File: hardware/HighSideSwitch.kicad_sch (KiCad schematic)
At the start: 5 parts, among them Q901 MMBTA42

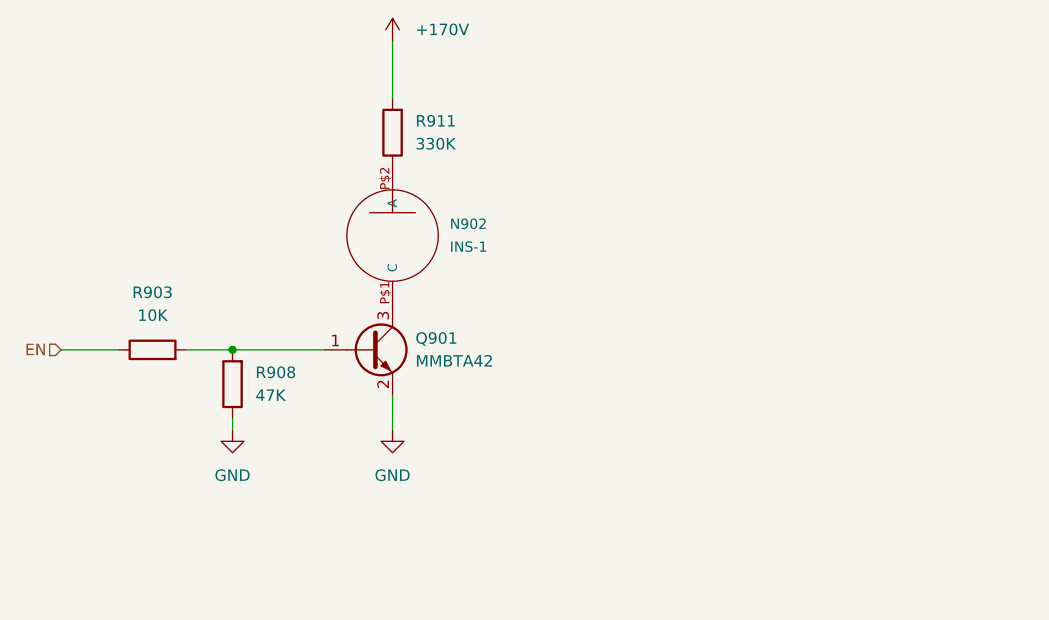
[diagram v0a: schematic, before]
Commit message: 2/static version
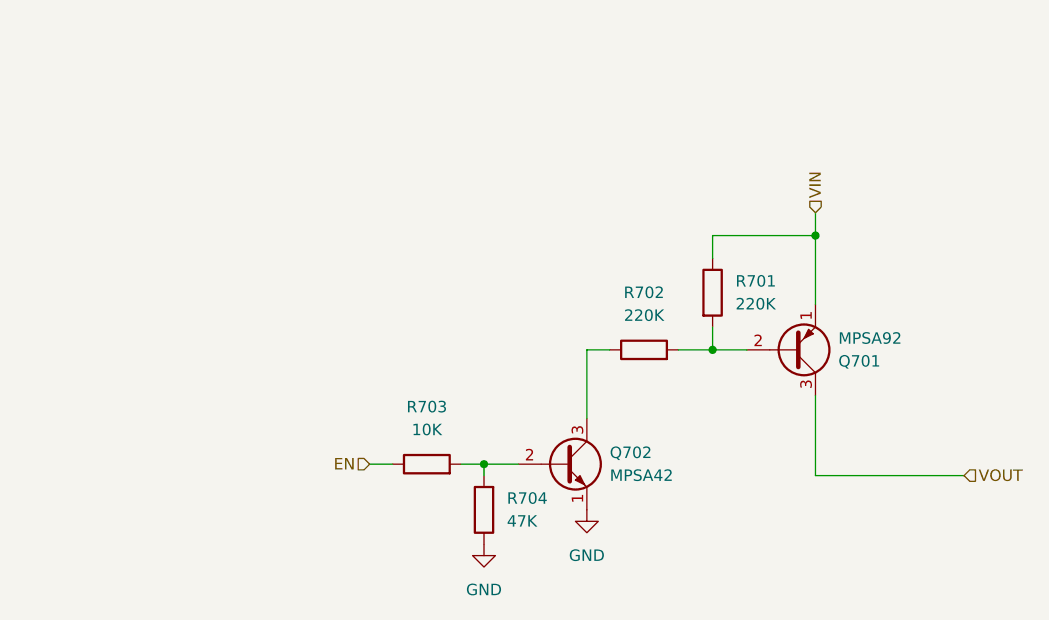
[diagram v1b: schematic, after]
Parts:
- removed N902: INS-1, mynixies:mynixies-INS-1, symbol mynixies:INS-1
- removed Q901: MMBTA42, Package_TO_SOT_SMD:SOT-23, symbol Transistor_BJT:MMBTA42
- removed R903: 10K, Resistor_SMD:R_0603_1608Metric, symbol Device:R
- removed R908: 47K, Resistor_SMD:R_0603_1608Metric, symbol Device:R
- removed R911: 330K, Resistor_SMD:R_1206_3216Metric, symbol Device:R
- added Q701: MPSA92, Package_TO_SOT_THT:TO-92_Inline, symbol Transistor_BJT:MPSA92
- added Q702: MPSA42, Package_TO_SOT_THT:TO-92_Inline, symbol Transistor_BJT:MPSA42
- added R701, R702: 220K, Resistor_SMD:R_1206_3216Metric, symbol Device:R
- added R703: 10K, Resistor_SMD:R_0603_1608Metric, symbol Device:R
- added R704: 47K, Resistor_SMD:R_0603_1608Metric, symbol Device:R
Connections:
- net EN: now also R703.1
- net GND: now also Q702.1 (E), R704.1
- new net: Q701.2 (B), R701.2, R702.2
- new net: Q702.3 (C), R702.1
- new net: Q702.2 (B), R703.2, R704.2
- new net VIN: Q701.1 (E), R701.1
- new net VOUT: Q701.3 (C)
